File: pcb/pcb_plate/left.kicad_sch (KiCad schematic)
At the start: 48 parts, among them J1 Conn_01x04, J2 Conn_01x04

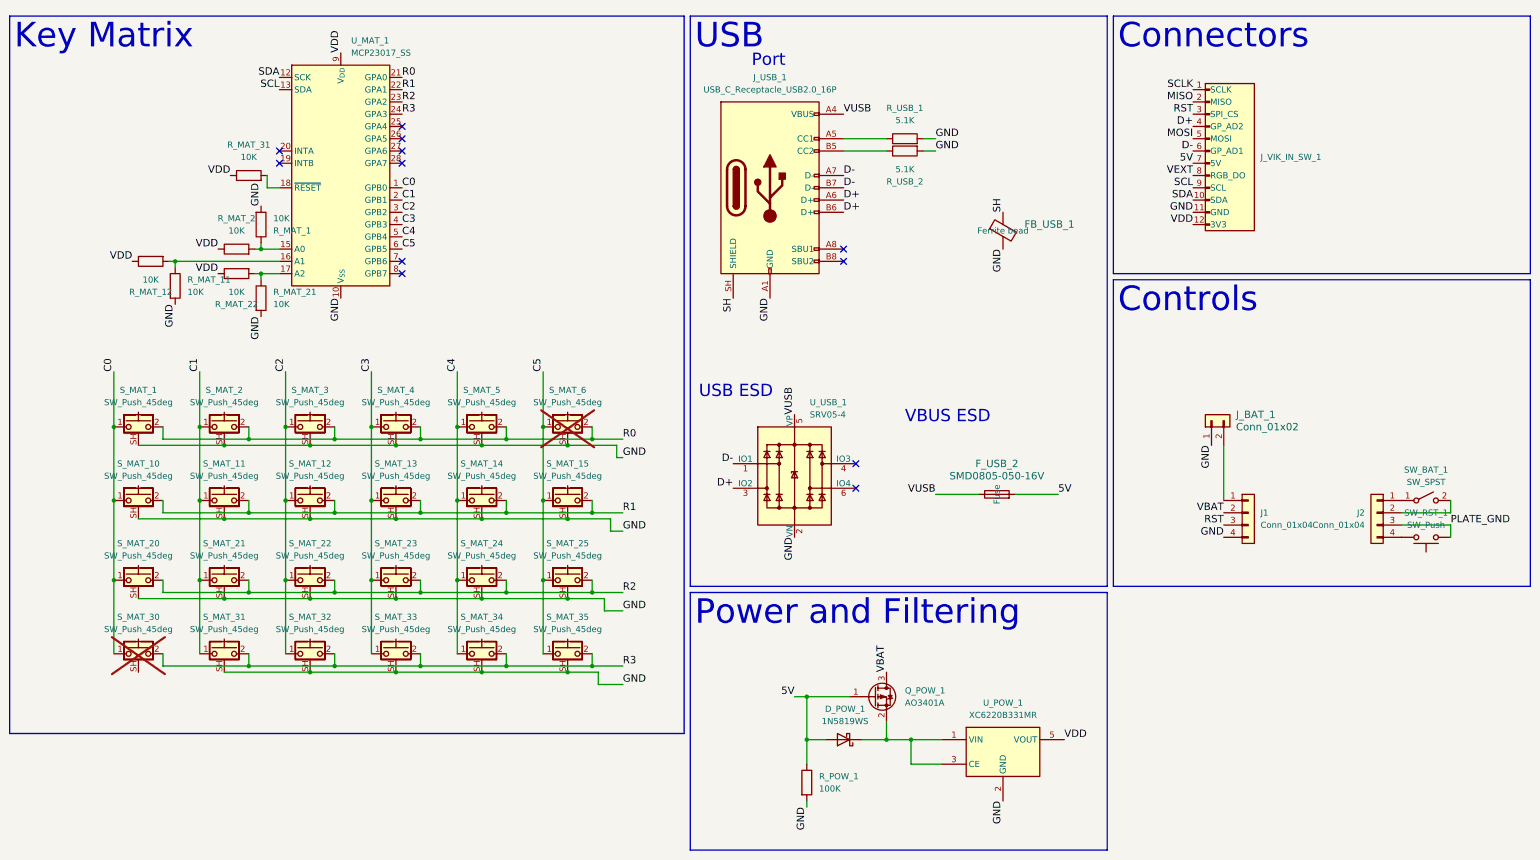
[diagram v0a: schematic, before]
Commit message: Redo matrix plates.
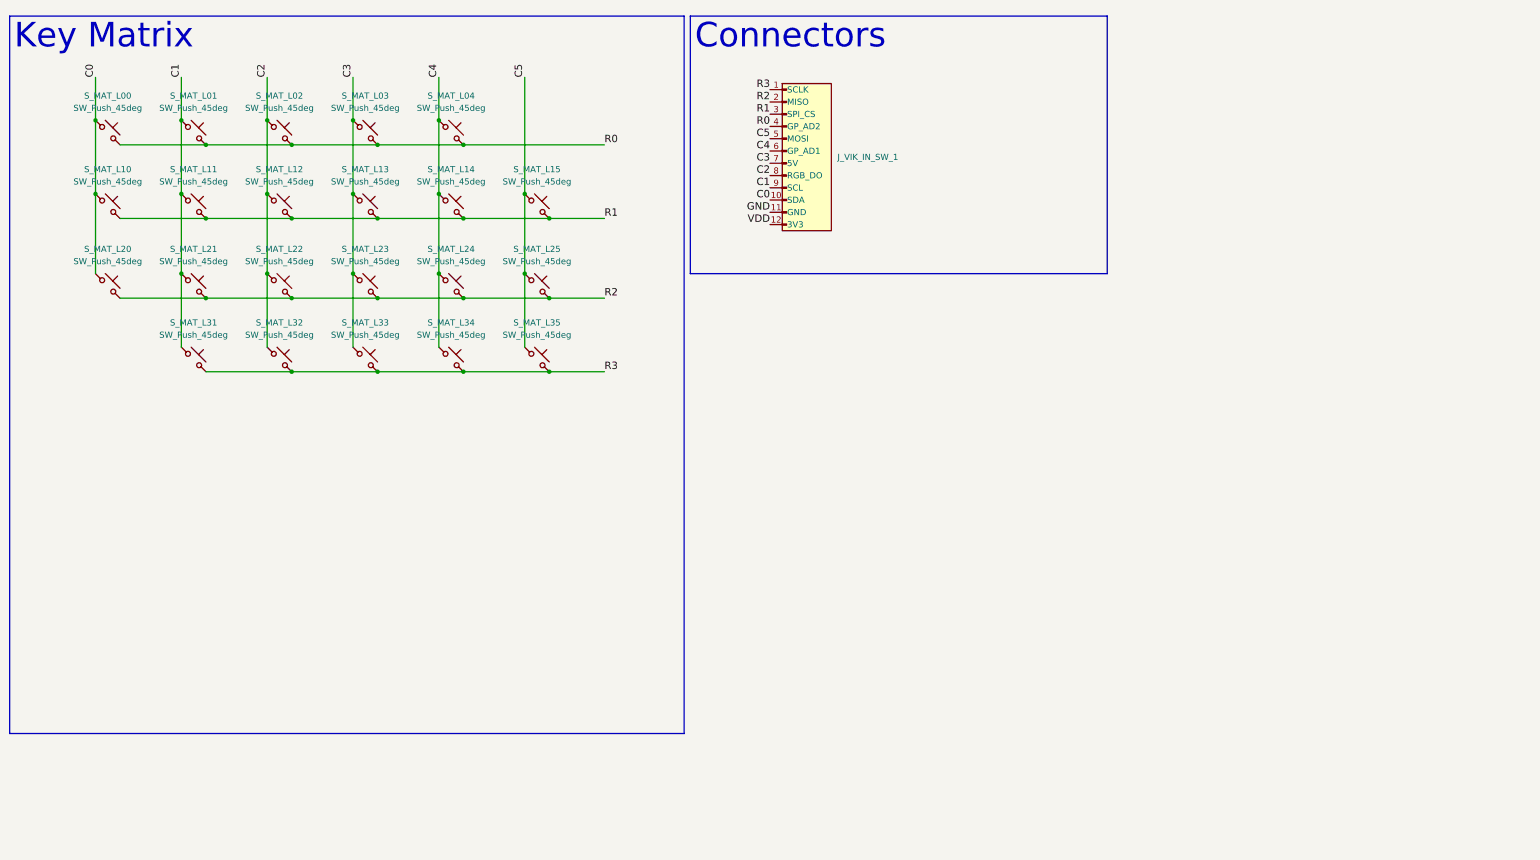
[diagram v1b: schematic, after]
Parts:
- removed D_POW_1: 1N5819WS, Diode_SMD:D_SOD-323, symbol Diode:1N5819WS
- removed FB_USB_1: (no value), Inductor_SMD:L_0805_2012Metric, symbol Device:FerriteBead
- removed F_USB_2: SMD0805-050-16V, Fuse:Fuse_0805_2012Metric, symbol Device:Fuse
- removed J1, J2: Conn_01x04, Connector_PinHeader_2.54mm:PinHeader_1x04_P2.54mm_Vertical, symbol Connector_Generic:Conn_01x04
- removed J_BAT_1: Conn_01x02, Connector_JST:JST_GH_SM02B-GHS-TB_1x02-1MP_P1.25mm_Horizontal, symbol Connector_Generic:Conn_01x02
- removed J_USB_1: USB_C_Receptacle_USB2.0_16P, Connector_USB:USB_C_Receptacle_HRO_TYPE-C-31-M-12, symbol Connector:USB_C_Receptacle_USB2.0_16P
- removed Q_POW_1: AO3401A, Package_TO_SOT_SMD:SOT-23, symbol Transistor_FET:AO3401A
- removed R_MAT_1, R_MAT_11, R_MAT_12, R_MAT_2, R_MAT_21, R_MAT_22, R_MAT_31: 10K, Resistor_SMD:R_0201_0603Metric_Pad0.64x0.40mm_HandSolder, symbol Device:R
- removed R_POW_1: 100K, Resistor_SMD:R_0201_0603Metric_Pad0.64x0.40mm_HandSolder, symbol Device:R
- removed R_USB_1, R_USB_2: 5.1K, Resistor_SMD:R_0201_0603Metric_Pad0.64x0.40mm_HandSolder, symbol Device:R
- removed SW_BAT_1: SW_SPST, library:AS11CH, symbol Switch:SW_SPST
- removed SW_RST_1: SW_Push, Button_Switch_SMD:SW_Push_1P1T_NO_E-Switch_TL3301NxxxxxG, symbol Switch:SW_Push
- removed S_MAT_30, S_MAT_6: SW_Push_45deg, key-switches:SW_Kailh_Choc_V1V2_HotSwap_PTH_Double, symbol Switch:SW_Push_Shielded
- removed U_MAT_1: MCP23017_SS, Package_SO:SSOP-28_5.3x10.2mm_P0.65mm, symbol Interface_Expansion:MCP23017x-x-SS
- removed U_POW_1: XC6220B331MR, Package_TO_SOT_SMD:SOT-23-5, symbol Regulator_Linear:XC6220B331MR
- removed U_USB_1: SRV05-4, Package_TO_SOT_SMD:SOT-23-6, symbol Power_Protection:SRV05-4
- S_MAT_L00: renamed from S_MAT_1; footprint key-switches:SW_Kailh_Choc_V1V2_HotSwap_PTH_Double -> key-switches:SW_GLP_Kailh_Choc_V1V2_HotSwap_PTH; symbol Switch:SW_Push_Shielded -> Switch:SW_Push_45deg
- S_MAT_L01: renamed from S_MAT_2; footprint key-switches:SW_Kailh_Choc_V1V2_HotSwap_PTH_Double -> key-switches:SW_GLP_Kailh_Choc_V1V2_HotSwap_PTH; symbol Switch:SW_Push_Shielded -> Switch:SW_Push_45deg
- S_MAT_L02: renamed from S_MAT_3; footprint key-switches:SW_Kailh_Choc_V1V2_HotSwap_PTH_Double -> key-switches:SW_GLP_Kailh_Choc_V1V2_HotSwap_PTH; symbol Switch:SW_Push_Shielded -> Switch:SW_Push_45deg
- S_MAT_L03: renamed from S_MAT_4; footprint key-switches:SW_Kailh_Choc_V1V2_HotSwap_PTH_Double -> key-switches:SW_GLP_Kailh_Choc_V1V2_HotSwap_PTH; symbol Switch:SW_Push_Shielded -> Switch:SW_Push_45deg
- S_MAT_L04: renamed from S_MAT_5; footprint key-switches:SW_Kailh_Choc_V1V2_HotSwap_PTH_Double -> key-switches:SW_GLP_Kailh_Choc_V1V2_HotSwap_PTH; symbol Switch:SW_Push_Shielded -> Switch:SW_Push_45deg
- S_MAT_L10: renamed from S_MAT_10; footprint key-switches:SW_Kailh_Choc_V1V2_HotSwap_PTH_Double -> key-switches:SW_GLP_Kailh_Choc_V1V2_HotSwap_PTH; symbol Switch:SW_Push_Shielded -> Switch:SW_Push_45deg
- S_MAT_L11: renamed from S_MAT_11; footprint key-switches:SW_Kailh_Choc_V1V2_HotSwap_PTH_Double -> key-switches:SW_GLP_Kailh_Choc_V1V2_HotSwap_PTH; symbol Switch:SW_Push_Shielded -> Switch:SW_Push_45deg
- S_MAT_L12: renamed from S_MAT_12; footprint key-switches:SW_Kailh_Choc_V1V2_HotSwap_PTH_Double -> key-switches:SW_GLP_Kailh_Choc_V1V2_HotSwap_PTH; symbol Switch:SW_Push_Shielded -> Switch:SW_Push_45deg
- S_MAT_L13: renamed from S_MAT_13; footprint key-switches:SW_Kailh_Choc_V1V2_HotSwap_PTH_Double -> key-switches:SW_GLP_Kailh_Choc_V1V2_HotSwap_PTH; symbol Switch:SW_Push_Shielded -> Switch:SW_Push_45deg
- S_MAT_L14: renamed from S_MAT_14; footprint key-switches:SW_Kailh_Choc_V1V2_HotSwap_PTH_Double -> key-switches:SW_GLP_Kailh_Choc_V1V2_HotSwap_PTH; symbol Switch:SW_Push_Shielded -> Switch:SW_Push_45deg
- S_MAT_L15: renamed from S_MAT_15; footprint key-switches:SW_Kailh_Choc_V1V2_HotSwap_PTH_Double -> key-switches:SW_GLP_Kailh_Choc_V1V2_HotSwap_PTH; symbol Switch:SW_Push_Shielded -> Switch:SW_Push_45deg
- S_MAT_L20: renamed from S_MAT_20; footprint key-switches:SW_Kailh_Choc_V1V2_HotSwap_PTH_Double -> key-switches:SW_GLP_Kailh_Choc_V1V2_HotSwap_PTH; symbol Switch:SW_Push_Shielded -> Switch:SW_Push_45deg
- S_MAT_L21: renamed from S_MAT_21; footprint key-switches:SW_Kailh_Choc_V1V2_HotSwap_PTH_Double -> key-switches:SW_GLP_Kailh_Choc_V1V2_HotSwap_PTH; symbol Switch:SW_Push_Shielded -> Switch:SW_Push_45deg
- S_MAT_L22: renamed from S_MAT_22; footprint key-switches:SW_Kailh_Choc_V1V2_HotSwap_PTH_Double -> key-switches:SW_GLP_Kailh_Choc_V1V2_HotSwap_PTH; symbol Switch:SW_Push_Shielded -> Switch:SW_Push_45deg
- S_MAT_L23: renamed from S_MAT_23; footprint key-switches:SW_Kailh_Choc_V1V2_HotSwap_PTH_Double -> key-switches:SW_GLP_Kailh_Choc_V1V2_HotSwap_PTH; symbol Switch:SW_Push_Shielded -> Switch:SW_Push_45deg
- S_MAT_L24: renamed from S_MAT_24; footprint key-switches:SW_Kailh_Choc_V1V2_HotSwap_PTH_Double -> key-switches:SW_GLP_Kailh_Choc_V1V2_HotSwap_PTH; symbol Switch:SW_Push_Shielded -> Switch:SW_Push_45deg
- S_MAT_L25: renamed from S_MAT_25; footprint key-switches:SW_Kailh_Choc_V1V2_HotSwap_PTH_Double -> key-switches:SW_GLP_Kailh_Choc_V1V2_HotSwap_PTH; symbol Switch:SW_Push_Shielded -> Switch:SW_Push_45deg
- S_MAT_L31: renamed from S_MAT_31; footprint key-switches:SW_Kailh_Choc_V1V2_HotSwap_PTH_Double -> key-switches:SW_GLP_Kailh_Choc_V1V2_HotSwap_PTH; symbol Switch:SW_Push_Shielded -> Switch:SW_Push_45deg
- S_MAT_L32: renamed from S_MAT_32; footprint key-switches:SW_Kailh_Choc_V1V2_HotSwap_PTH_Double -> key-switches:SW_GLP_Kailh_Choc_V1V2_HotSwap_PTH; symbol Switch:SW_Push_Shielded -> Switch:SW_Push_45deg
- S_MAT_L33: renamed from S_MAT_33; footprint key-switches:SW_Kailh_Choc_V1V2_HotSwap_PTH_Double -> key-switches:SW_GLP_Kailh_Choc_V1V2_HotSwap_PTH; symbol Switch:SW_Push_Shielded -> Switch:SW_Push_45deg
- S_MAT_L34: renamed from S_MAT_34; footprint key-switches:SW_Kailh_Choc_V1V2_HotSwap_PTH_Double -> key-switches:SW_GLP_Kailh_Choc_V1V2_HotSwap_PTH; symbol Switch:SW_Push_Shielded -> Switch:SW_Push_45deg
- S_MAT_L35: renamed from S_MAT_35; footprint key-switches:SW_Kailh_Choc_V1V2_HotSwap_PTH_Double -> key-switches:SW_GLP_Kailh_Choc_V1V2_HotSwap_PTH; symbol Switch:SW_Push_Shielded -> Switch:SW_Push_45deg
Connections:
- net 5V is gone; now on net C3: J_VIK_IN_SW_1.7 (5V)
- net D+ is gone; now on net R0: J_VIK_IN_SW_1.4 (GP_AD2)
- net D- is gone; now on net C4: J_VIK_IN_SW_1.6 (GP_AD1)
- net MISO is gone; now on net R2: J_VIK_IN_SW_1.2 (MISO)
- net MOSI is gone; now on net C5: J_VIK_IN_SW_1.5 (MOSI)
- net RST is gone; now on net R1: J_VIK_IN_SW_1.3 (SPI_CS)
- net SCL is gone; now on net C1: J_VIK_IN_SW_1.9 (SCL)
- net SCLK is gone; now on net R3: J_VIK_IN_SW_1.1 (SCLK)
- net SDA is gone; now on net C0: J_VIK_IN_SW_1.10 (SDA)
- net VEXT is gone; now on net C2: J_VIK_IN_SW_1.8 (RGB_DO)
- net GND: no longer S_MAT_L00.SH (B), S_MAT_L01.SH (B), S_MAT_L02.SH (B), S_MAT_L03.SH (B), S_MAT_L04.SH (B), S_MAT_L10.SH (B), S_MAT_L11.SH (B), S_MAT_L12.SH (B), S_MAT_L13.SH (B), S_MAT_L14.SH (B), S_MAT_L15.SH (B), S_MAT_L20.SH (B), S_MAT_L21.SH (B), S_MAT_L22.SH (B), S_MAT_L23.SH (B), S_MAT_L24.SH (B), S_MAT_L25.SH (B), S_MAT_L31.SH (B), S_MAT_L32.SH (B), S_MAT_L33.SH (B), S_MAT_L34.SH (B), S_MAT_L35.SH (B)
- no-connect marks 12 -> 0
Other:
- note removed: "Port"
- note removed: "USB ESD"
- note removed: "VBUS ESD"
- moved on the sheet: J_VIK_IN_SW_1
